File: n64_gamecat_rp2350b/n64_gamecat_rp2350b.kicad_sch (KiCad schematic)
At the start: 6 parts, among them J1 Conn_01x03_Pin, J2 Conn_01x03_Pin, J3 Conn_01x05, U4 RP235x-B

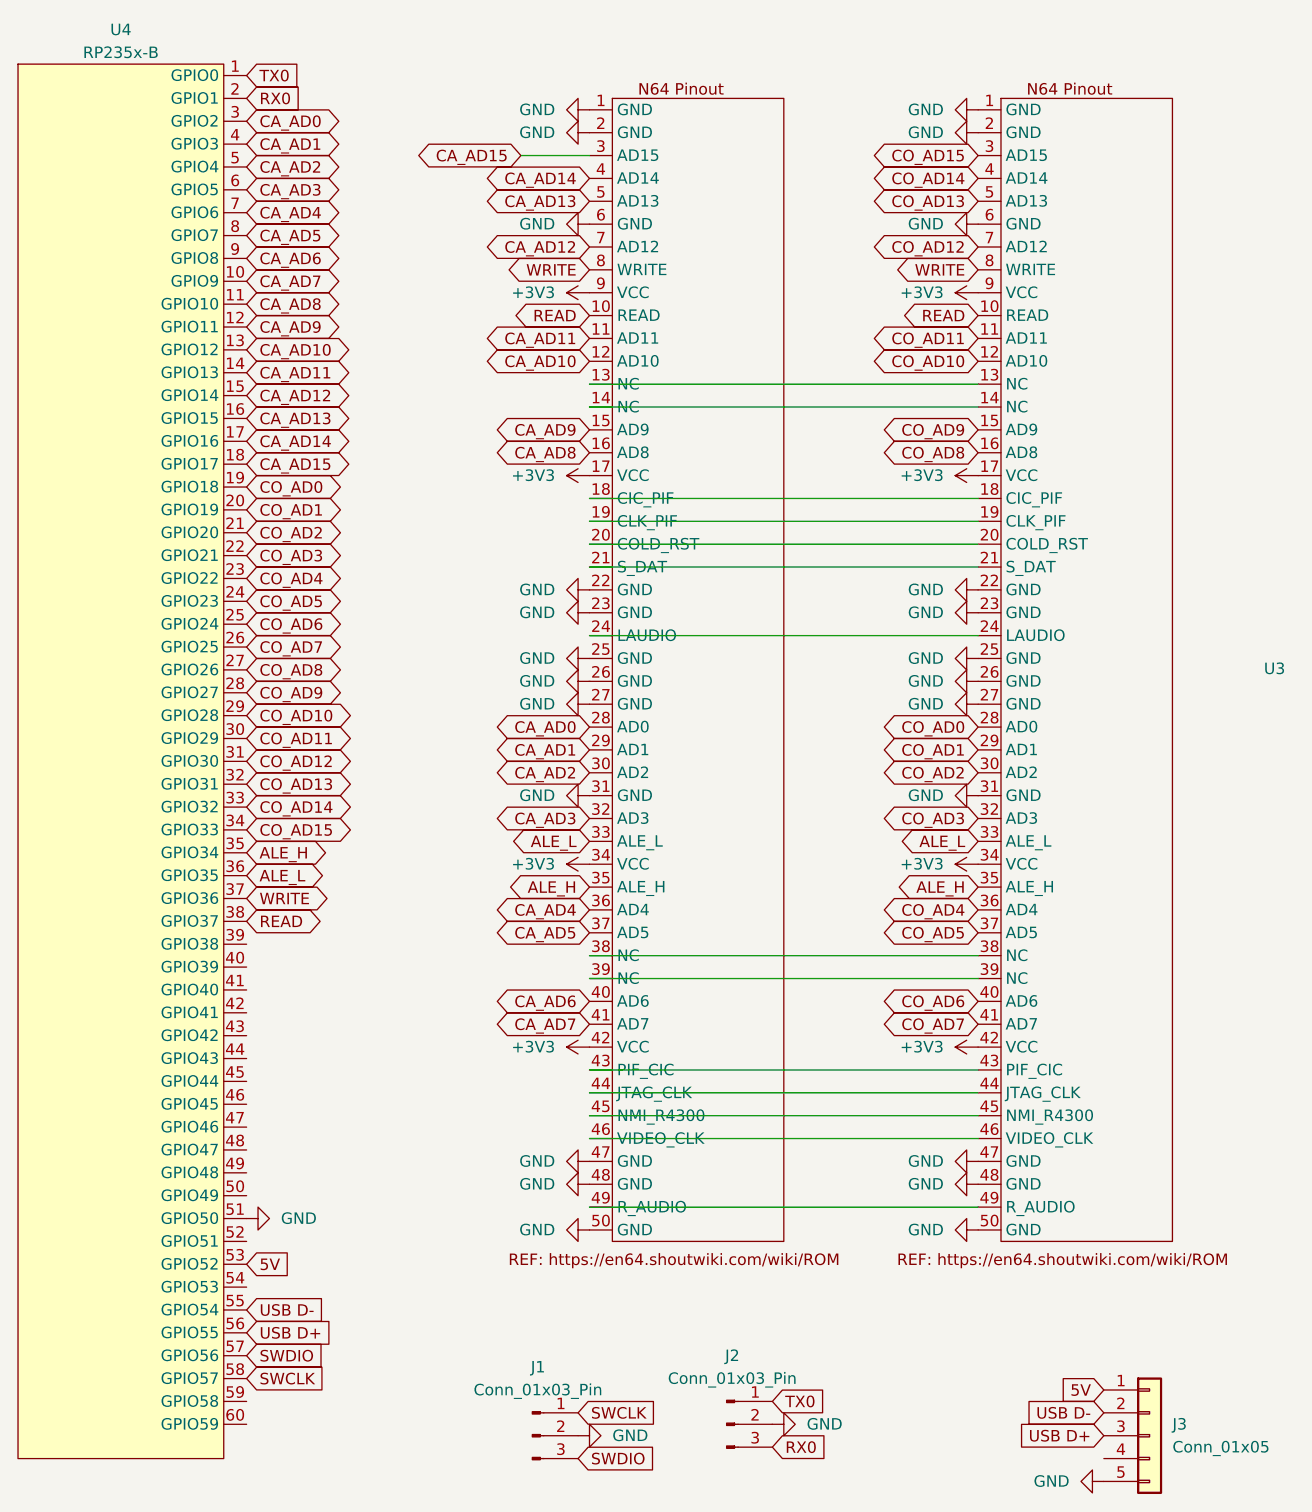
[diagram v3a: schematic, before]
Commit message: Add v0.9 PCB
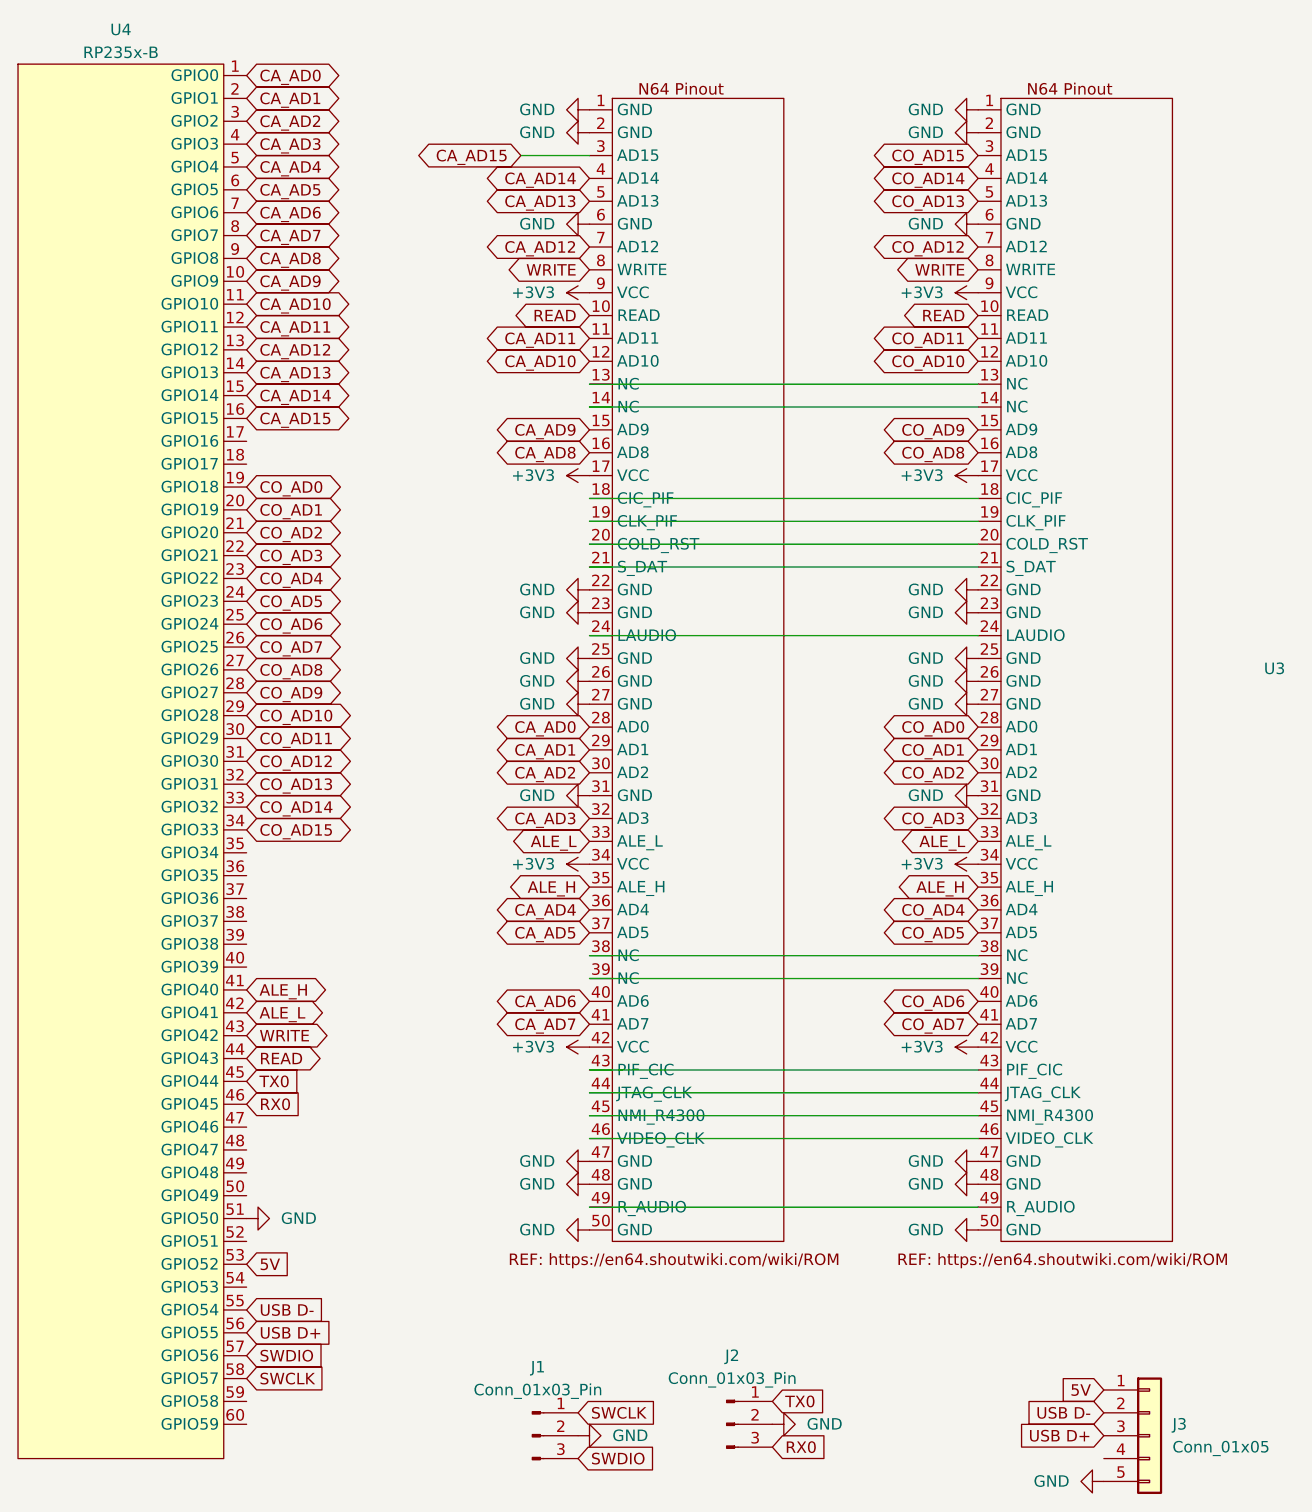
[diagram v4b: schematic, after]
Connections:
- net ALE_H: now also U4.41 (GPIO40); no longer U4.35 (GPIO34)
- net ALE_L: now also U4.42 (GPIO41); no longer U4.36 (GPIO35)
- net CA_AD0: now also U4.1 (GPIO0); no longer U4.3 (GPIO2)
- net CA_AD1: now also U4.2 (GPIO1); no longer U4.4 (GPIO3)
- net CA_AD10: now also U4.11 (GPIO10); no longer U4.13 (GPIO12)
- net CA_AD11: now also U4.12 (GPIO11); no longer U4.14 (GPIO13)
- net CA_AD12: now also U4.13 (GPIO12); no longer U4.15 (GPIO14)
- net CA_AD13: now also U4.14 (GPIO13); no longer U4.16 (GPIO15)
- net CA_AD14: now also U4.15 (GPIO14); no longer U4.17 (GPIO16)
- net CA_AD15: now also U4.16 (GPIO15); no longer U4.18 (GPIO17)
- net CA_AD2: now also U4.3 (GPIO2); no longer U4.5 (GPIO4)
- net CA_AD3: now also U4.4 (GPIO3); no longer U4.6 (GPIO5)
- net CA_AD4: now also U4.5 (GPIO4); no longer U4.7 (GPIO6)
- net CA_AD5: now also U4.6 (GPIO5); no longer U4.8 (GPIO7)
- net CA_AD6: now also U4.7 (GPIO6); no longer U4.9 (GPIO8)
- net CA_AD7: now also U4.8 (GPIO7); no longer U4.10 (GPIO9)
- net CA_AD8: now also U4.9 (GPIO8); no longer U4.11 (GPIO10)
- net CA_AD9: now also U4.10 (GPIO9); no longer U4.12 (GPIO11)
- net READ: now also U4.44 (GPIO43); no longer U4.38 (GPIO37)
- net RX0: now also U4.46 (GPIO45); no longer U4.2 (GPIO1)
- net TX0: now also U4.45 (GPIO44); no longer U4.1 (GPIO0)
- net WRITE: now also U4.43 (GPIO42); no longer U4.37 (GPIO36)
